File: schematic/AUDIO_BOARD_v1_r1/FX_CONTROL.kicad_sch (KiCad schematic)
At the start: 6 parts, among them J20 FX-CTRL FFC, U20 DAC8565

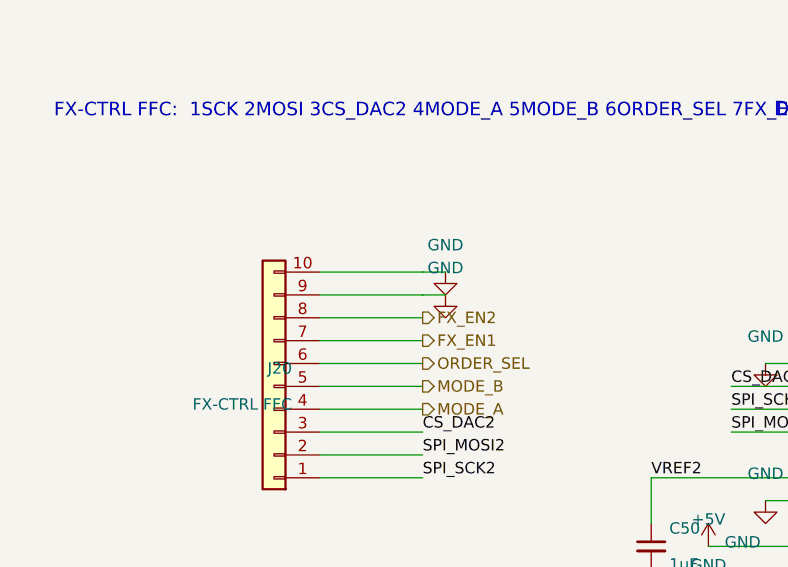
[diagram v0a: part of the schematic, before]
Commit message: working on chorus and phaser
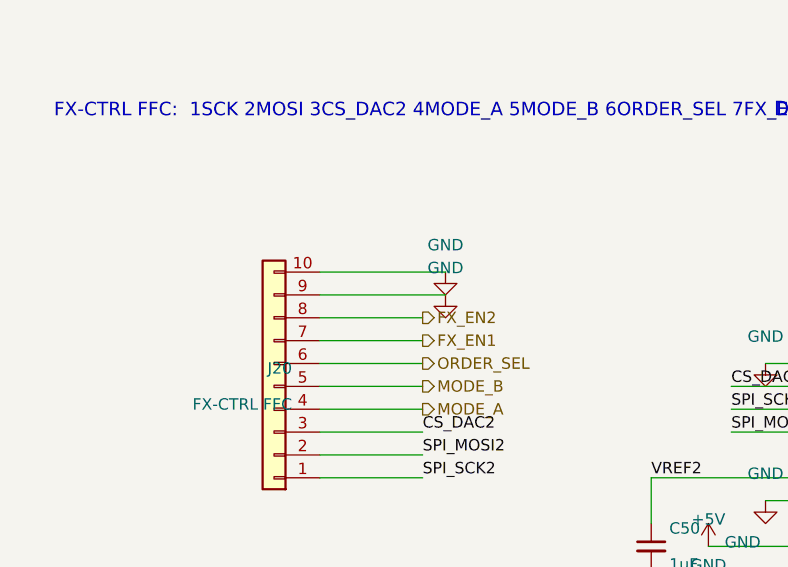
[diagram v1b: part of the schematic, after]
